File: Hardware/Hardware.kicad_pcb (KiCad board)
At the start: 2 copper layers, 50 x 50 mm, 42 parts, among them J1 USB4105-GF-A, J2 Conn_01x06_Socket, J3 Conn_01x06_Socket, SW1 SW_Push, SW2 SW_Push, U1 ESP32-C3-MINI-1-N4, U3 LM1117MP-3.3

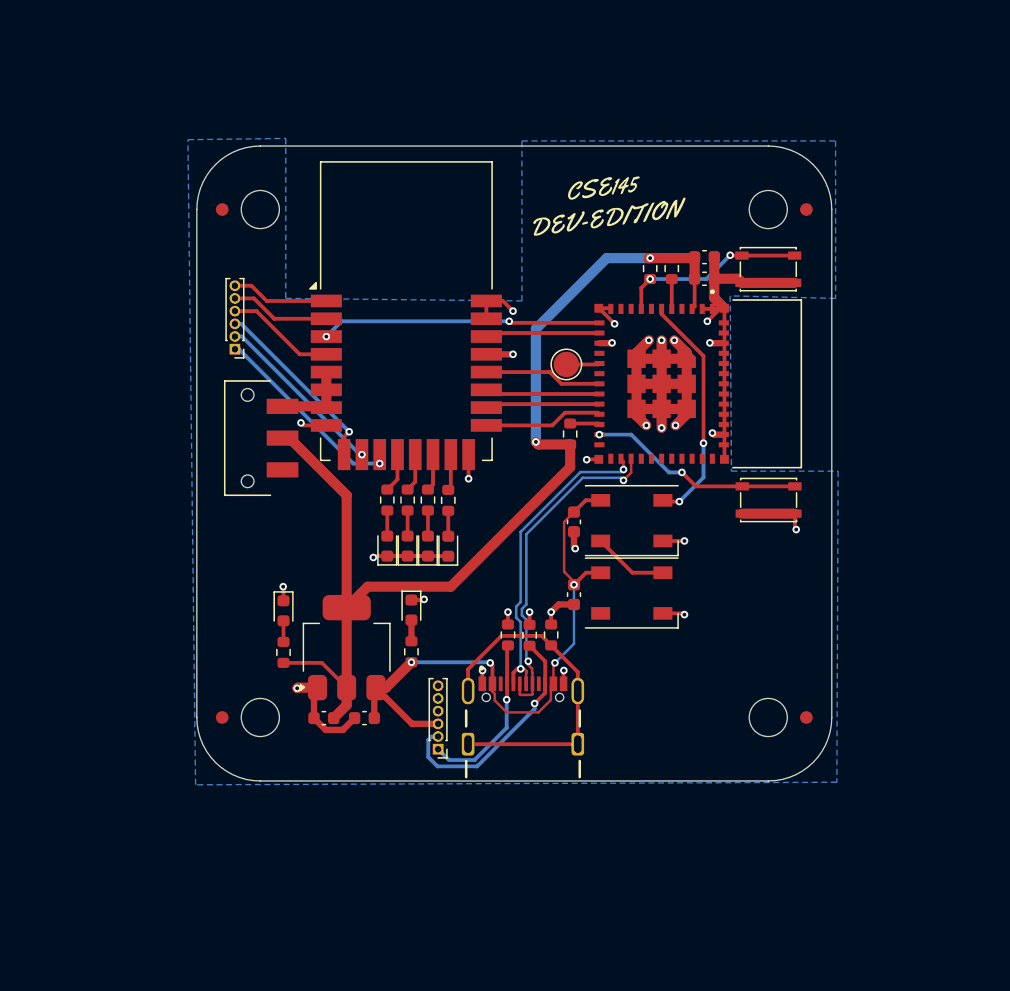
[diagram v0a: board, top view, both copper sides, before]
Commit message: hardware updates
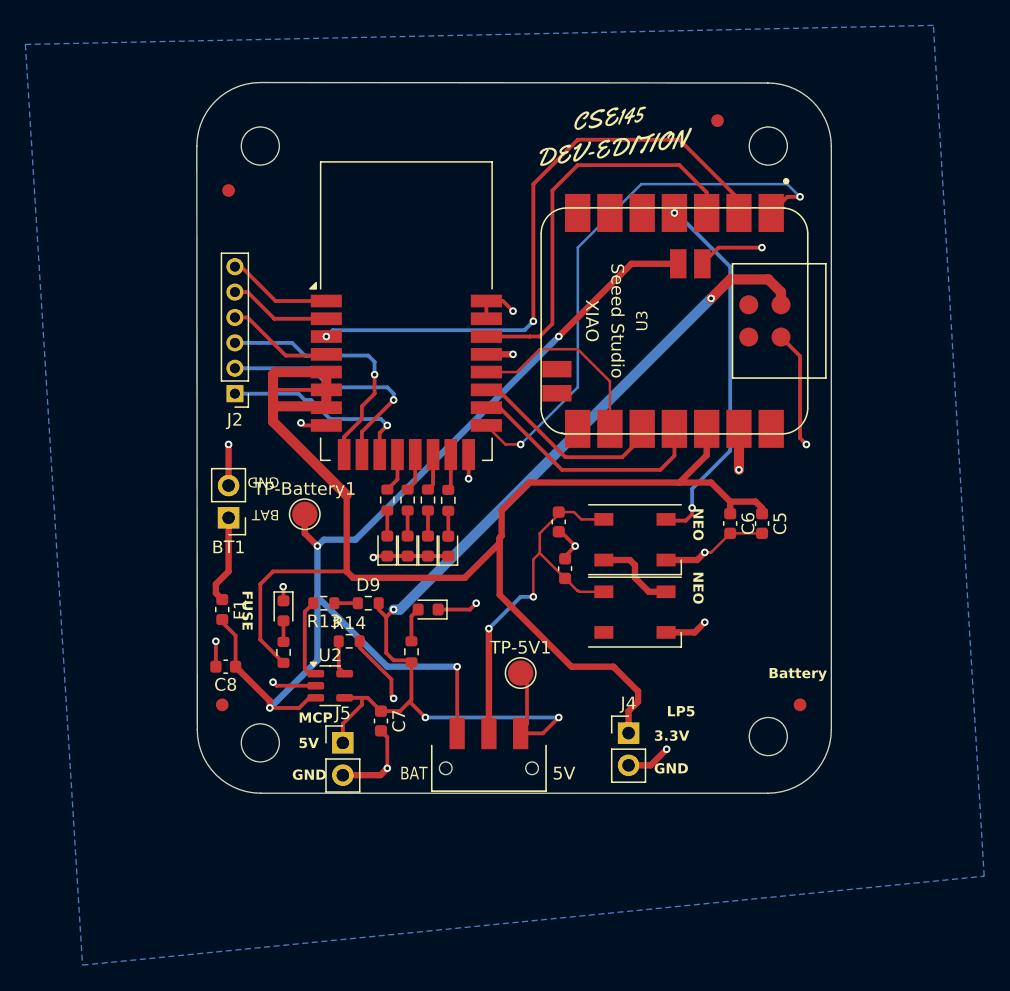
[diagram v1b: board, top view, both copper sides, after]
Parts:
- removed C1: 10u, Capacitor_SMD:C_0603_1608Metric
- removed C2: .1u, Capacitor_SMD:C_0603_1608Metric
- removed J1: USB4105-GF-A, opentags_library:GCT_USB4105-GF-A
- removed J3: Conn_01x06_Socket, Connector_PinHeader_1.00mm:PinHeader_1x06_P1.00mm_Vertical
- removed R1: 100K, Resistor_SMD:R_0603_1608Metric
- removed R10: 50k, Resistor_SMD:R_0603_1608Metric
- removed R2, R3: 5k1, Resistor_SMD:R_0603_1608Metric
- removed R8, R9: 10k, Resistor_SMD:R_0603_1608Metric
- removed S1: JS102011SAQN, opentags_library:SW_JS102011SAQN
- removed SW2: SW_Push, Button_Switch_SMD:SW_SPST_PTS810
- removed TP1: TestPoint, TestPoint:TestPoint_Pad_D2.0mm
- removed U1: ESP32-C3-MINI-1-N4, opentags_library:XCVR_ESP32-C3-MINI-1-N4
- added BT1: Battery_Cell, Connector_PinHeader_2.54mm:PinHeader_1x02_P2.54mm_Vertical, F.Cu at (102.5, 74.3)
- added C7: 4.7u, Capacitor_SMD:C_0603_1608Metric, F.Cu at (114.5, 90.3)
- added C8: 4.7u, Capacitor_SMD:C_0603_1608Metric, F.Cu at (102.3, 86.0)
- added D9: LED, Resistor_SMD:R_0603_1608Metric, F.Cu at (113.5, 81.0)
- added F1: 1 Amp Fuse, Fuse:Fuse_0603_1608Metric, F.Cu at (102.0, 81.5)
- added J4: Conn_01x02_Socket, Connector_PinHeader_2.54mm:PinHeader_1x02_P2.54mm_Vertical, F.Cu at (134.0, 91.2)
- added J5: Conn_01x02_Socket, Connector_PinHeader_2.54mm:PinHeader_1x02_P2.54mm_Vertical, F.Cu at (111.5, 92.0)
- added R13: 470, Resistor_SMD:R_0603_1608Metric, F.Cu at (110.0, 81.0)
- added R14: 2.5k, Resistor_SMD:R_0603_1608Metric, F.Cu at (112.0, 84.0)
- added TP-5V1: TestPoint, TestPoint:TestPoint_Pad_D2.0mm, F.Cu at (125.5, 86.5)
- added TP-Battery1: TestPoint, TestPoint:TestPoint_Pad_D2.0mm, F.Cu at (108.5, 74.0)
- added U2: MCP73831-5-OT, Package_TO_SOT_SMD:SOT-23-5, F.Cu at (110.5, 87.5)
- C6: value 10u -> .1u
- J2: footprint Connector_PinHeader_1.00mm:PinHeader_1x06_P1.00mm_Vertical -> Connector_PinHeader_2.00mm:PinHeader_1x06_P2.00mm_Vertical
- SW1: value SW_Push -> SW_SPST; footprint Button_Switch_SMD:SW_SPST_PTS810 -> opentags_library:SW_JS102011SAQN
- U3: value LM1117MP-3.3 -> Seeed Studio XIAO SAMD21; footprint Package_TO_SOT_SMD:SOT-223-3_TabPin2 -> Seeed Studio XIAO Series Library:XIAO-nRF52840-Sense-14P-2.54-21X17.8MM
- moved SW1 45.0 mm to (123.0, 94.0)
- moved U3 36.4 mm to (137.6, 58.8), turned to -90 degrees
- moved C6 35.5 mm to (142.0, 74.7), turned to -90 degrees
- moved C5 34.9 mm to (144.5, 74.7), turned to -90 degrees
- moved FID2 9.90 mm to (141.0, 43.0)
- moved G*** 5.52 mm to (132.5, 44.0)
- moved J2 3.50 mm to (103.0, 64.5)
- moved C4 2.17 mm to (129.0, 78.3), turned to -90 degrees
- moved FID1 1.58 mm to (102.5, 48.5)
- moved D5 1.52 mm to (134.5, 76.0)
- moved D6 1.52 mm to (134.5, 81.7)
- moved D7 1.31 mm to (118.2, 81.5), turned to 180 degrees
- moved C3 1.20 mm to (128.5, 74.6)
- moved FID4 1.12 mm to (147.5, 89.0)
- moved FID3 1.00 mm to (102.0, 89.0)
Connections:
- C3 pad 2: +5V -> Voltage Source
- C4 pad 2: +5V -> Voltage Source
- C5 pad 1: +5V -> +3.3V
- D5 pad 3: +5V -> Voltage Source
- D6 pad 3: +5V -> Voltage Source
- DWM1 pad 5: Net-(DWM1-VDDAON) -> +3.3V
- DWM1 pad 6: Net-(DWM1-VDDAON) -> +3.3V
- DWM1 pad 7: Net-(DWM1-VDDAON) -> +3.3V
- SW1 pad 1: Net-(U1-EN) -> +BATT
- SW1 pad 2: GND -> Voltage Source
- U3 pad 1: GND -> /DWM3000_SPICS
- U3 pad 2: +3.3V -> /DWM3000_RSTn
- U3 pad 3: +5V -> /DWM3000_IRQ
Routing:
- net +BATT: track 0.00 -> 85.0 mm, vias 0 -> 4
- net +5V: track 47.9 -> 84.1 mm
- net /DWM3000_SPICS: track 9.37 -> 43.5 mm, vias 0 -> 2
- net GND: track 112.4 -> 78.5 mm, vias 29 -> 19
- net Voltage Source: track 0.00 -> 30.3 mm, vias 0 -> 2
- net +3.3V: track 87.0 -> 114.1 mm, vias 2 -> 0
- net Net-(J1-SHELL_GND-PadSH1): track 26.9 -> 0.00 mm
- net /DP: track 26.5 -> 0.00 mm, vias 2 -> 0
- net /DWM3000_RSTn: track 22.0 -> 48.3 mm
- net /DN: track 25.3 -> 0.00 mm, vias 2 -> 0
- net /DWM3000_IRQ: track 9.01 -> 31.6 mm
- net /CC2: track 18.6 -> 0.00 mm, vias 1 -> 0
- net Net-(U1-IO9): track 17.1 -> 0.00 mm, vias 2 -> 0
- net Net-(U1-EN): track 14.8 -> 0.00 mm, vias 2 -> 0
- net /CC1: track 13.3 -> 0.00 mm, vias 1 -> 0
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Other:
- board size 50 x 50 mm -> 50 x 56 mm
- board text added: "3.3V GND"
- board text added: "5V"
- board text added: "BAT"
- board text added: "BAT GND"
- board text added: "Battery"
- board text added: "FUSE"
- board text added: "GND"
- board text added: "LP5"
- board text added: "MCP"
- board text added: "NEO"
